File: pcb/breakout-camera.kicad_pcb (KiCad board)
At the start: 2 copper layers, 50 x 50 mm, 64 parts, among them P10 OUTP, P4 HORI, P5 OUTP, P6 POWER, P7 VERT, Q1 2SC5095, Q2 MT3S20TU, Q3 2SC5095, Q4 MT3S20TU, U10 ICX825AQA, U4 TXB0104, U5 ADDI9023, U6 ADA4800, U9 ADA4800

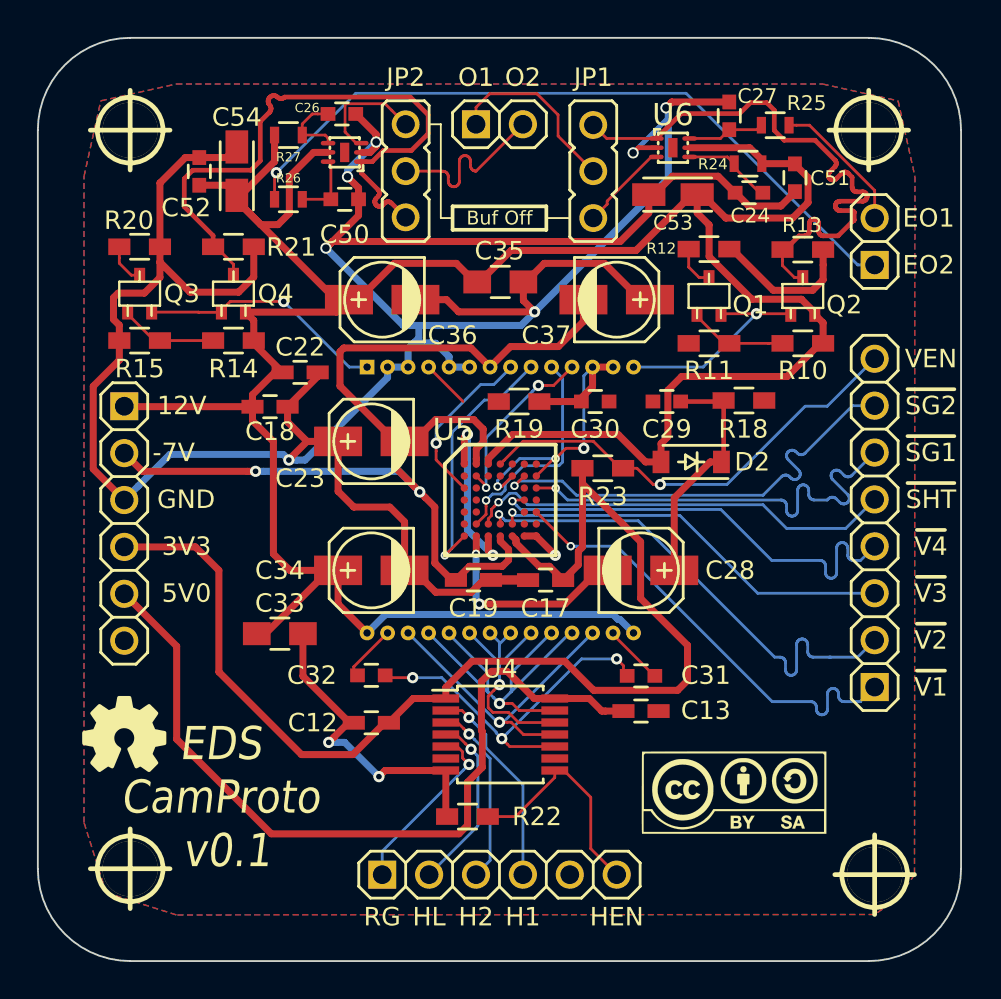
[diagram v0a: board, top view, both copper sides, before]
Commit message: ready for ordering
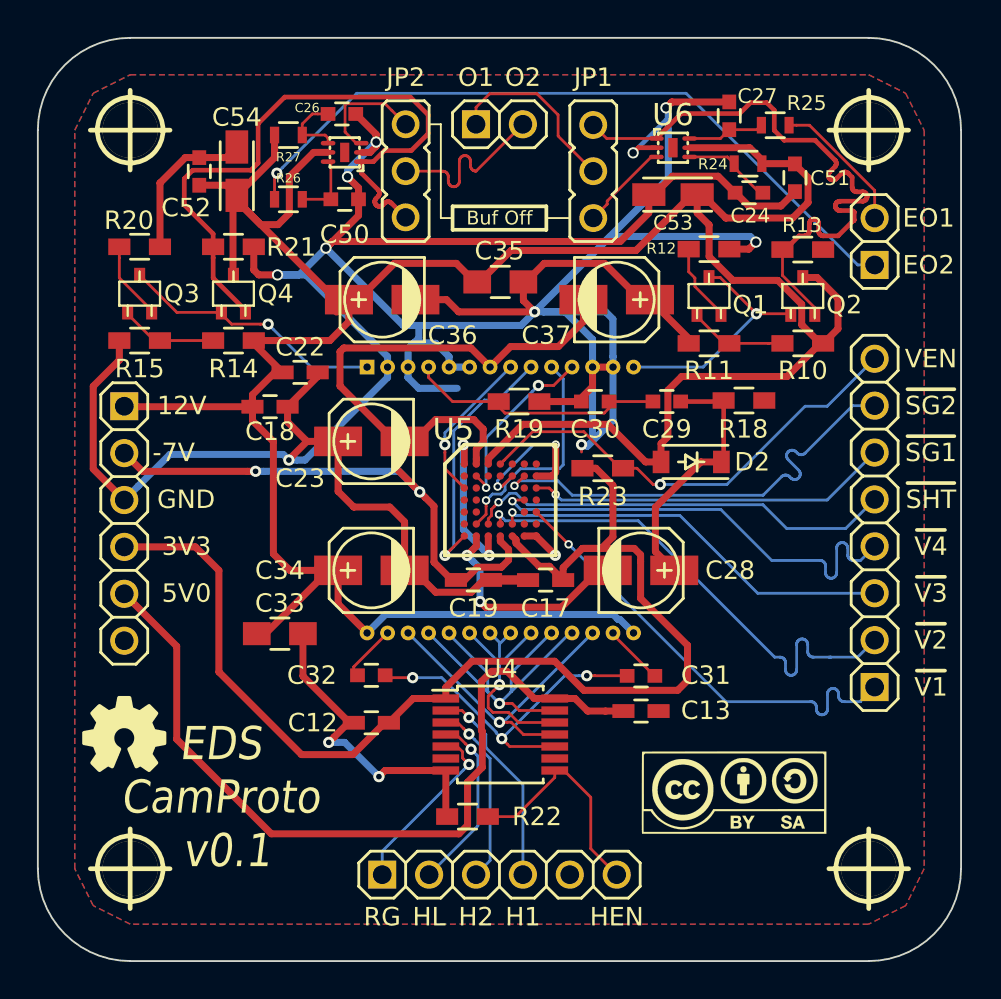
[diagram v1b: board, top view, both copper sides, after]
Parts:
- moved hole_3mm 0.45 mm to (96.2, 83.5)
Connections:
- Q1 pad 2: /camera/E1 -> /camera/VOUT1
- Q1 pad 3: /camera/VOUT1 -> /camera/E1
- Q2 pad 2: /camera/VO1 -> /camera/12V
- Q2 pad 3: /camera/12V -> /camera/VO1
- Q3 pad 2: /camera/E2 -> /camera/VOUT2
- Q3 pad 3: /camera/VOUT2 -> /camera/E2
- Q4 pad 2: /camera/VO2 -> /camera/12V
- Q4 pad 3: /camera/12V -> /camera/VO2
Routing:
- net GND: track 231.3 -> 255.0 mm, vias 15 -> 17
- net /camera/SUB: track 2.64 -> 14.2 mm
- net /camera/12V: track 154.2 -> 164.0 mm
- net /camera/XSGV2: track 25.0 -> 19.7 mm
- net /camera/E1: track 2.31 -> 4.32 mm
- net /camera/E2: track 2.26 -> 4.27 mm
- net /camera/VO1: track 32.3 -> 34.3 mm
- net /camera/VO2: track 33.9 -> 35.6 mm
- net /camera/VOUT1: track 11.8 -> 13.2 mm
- net /camera/VOUT2: track 13.4 -> 14.6 mm
- net /camera/SCKP: track 13.1 -> 14.2 mm
- net /camera/ORG: track 19.7 -> 18.6 mm
- net /camera/VT1: track 9.27 -> 8.46 mm
- net /camera/3V3: track 65.3 -> 65.8 mm
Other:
- rule pad_to_mask_clearance: 0 -> 0.0635
